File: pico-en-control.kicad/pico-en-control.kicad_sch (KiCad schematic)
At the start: 17 parts, among them J1 JST-PH2 Bat, J2 Pico Pin 1-13, J3 Pico Pin 40-28, SW1 SW_Push, U1 SN74HC74N, U2 PCF8563T, Y1 Crystal

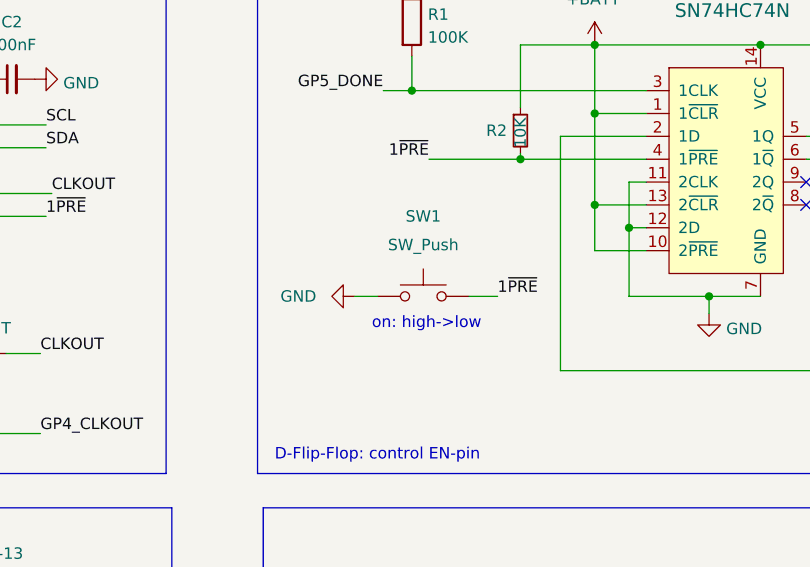
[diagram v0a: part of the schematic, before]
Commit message: Rev2
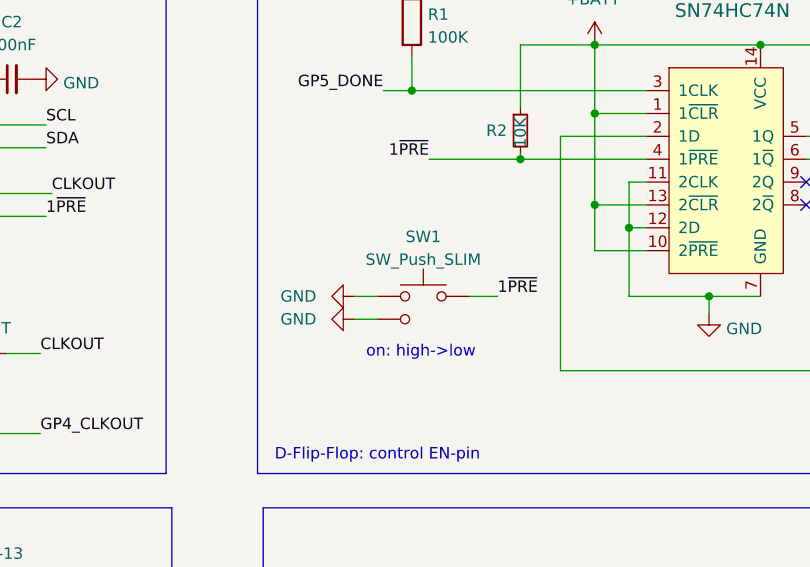
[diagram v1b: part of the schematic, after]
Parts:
- removed SW1: SW_Push, user:SW_PUSH_SLIM_1x4, symbol Switch:SW_Push
- added SW1: SW_Push_SLIM, user:SW_PUSH_SLIM_1x4, symbol user:SW_Push_SLIM
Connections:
- net 1~{PRE}: now also SW1.2
- net GND: now also SW1.1, SW1.3 (1)
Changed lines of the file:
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@@
+    (stroke (width 0) (type default) (color 0 0 0 0))
+  )
+  (wire (pts (xy 161.925 77.47) (xy 164.465 77.47))
     (stroke (width 0) (type default) (color 0 0 0 0))
   )
@@
     (effects (font (size 1.27 1.27)) (justify left bottom))
   )
-  (text "on: high->low" (at 163.83 78.74 0)
+  (text "on: high->low" (at 163.195 81.915 0)
     (effects (font (size 1.27 1.27)) (justify left bottom))
   )
@@
   (symbol (lib_id "power:GND") (at 123.825 137.795 90) (mirror x) (unit 1)
     (in_bom yes) (on_board yes)
-    (property "Reference" "#PWR?" (id 0) (at 130.175 137.795 0)
+    (property "Reference" "#PWR0107" (id 0) (at 130.175 137.795 0)
       (effects (font (size 1.27 1.27)) hide)
     )
@@
     (pin "1")
   )
+  (symbol (lib_id "power:GND") (at 161.925 77.47 270) (unit 1)
+    (in_bom yes) (on_board yes)
+    (property "Reference" "#PWR0110" (id 0) (at 155.575 77.47 0)
+      (effects (font (size 1.27 1.27)) hide)
+    )
+    (property "Value" "GND" (id 1) (at 153.67 77.47 90)
+      (effects (font (size 1.27 1.27)) (justify left))
+    )
+    (property "Footprint" "" (id 2) (at 161.925 77.47 0)
+      (effects (font (size 1.27 1.27)) hide)
+    )
+    (property "Datasheet" "" (id 3) (at 161.925 77.47 0)
+      (effects (font (size 1.27 1.27)) hide)
+    )
+    (pin "1")
+  )
   (symbol (lib_id "power:PWR_FLAG") (at 214.63 118.11 270) (unit 1)
     (in_bom yes) (on_board yes) (fields_autoplaced)
@@
   (symbol (lib_id "power:GND") (at 85.09 138.43 270) (unit 1)
     (in_bom yes) (on_board yes)
-    (property "Reference" "#PWR?" (id 0) (at 78.74 138.43 0)
+    (property "Reference" "#PWR0108" (id 0) (at 78.74 138.43 0)
       (effects (font (size 1.27 1.27)) hide)
     )
@@
     (pin "1")
   )
+  (symbol (lib_id "user:SW_Push_SLIM") (at 169.545 74.93 0) (unit 1)
+    (in_bom yes) (on_board yes) (fields_autoplaced)
+    (property "Reference" "SW1" (id 0) (at 169.545 68.3092 0))
+    (property "Value" "SW_Push_SLIM" (id 1) (at 169.545 70.8461 0))
+    (property "Footprint" "user:SW_PUSH_SLIM_1x4" (id 2) (at 169.545 82.55 0)
+      (effects (font (size 1.27 1.27)) hide)
+    )
+    (property "Datasheet" "" (id 3) (at 169.545 69.85 0)
+      (effects (font (size 1.27 1.27)) hide)
+    )
+    (pin "1")
+    (pin "2")
+    (pin "3")
+  )
   (symbol (lib_id "Device:C_Small") (at 218.44 46.99 90) (unit 1)
     (in_bom yes) (on_board yes)
@@
     )
     (property "LCSC" "C25744" (id 4) (at 90.17 82.55 0)
-      (effects (font (size 1.27 1.27)) hide)
-    )
-    (pin "1")
-    (pin "2")
-  )
-  (symbol (lib_id "Switch:SW_Push") (at 169.545 74.93 0) (unit 1)
-    (in_bom yes) (on_board yes)
-    (property "Reference" "SW1" (id 0) (at 169.545 66.04 0))
-    (property "Value" "SW_Push" (id 1) (at 169.545 69.215 0))
-    (property "Footprint" "user:SW_PUSH_SLIM_1x4" (id 2) (at 169.545 69.85 0)
-      (effects (font (size 1.27 1.27)) hide)
-    )
-    (property "Datasheet" "~" (id 3) (at 169.545 69.85 0)
       (effects (font (size 1.27 1.27)) hide)
     )
@@
   (symbol (lib_id "power:GND") (at 85.09 125.73 270) (unit 1)
     (in_bom yes) (on_board yes)
-    (property "Reference" "#PWR?" (id 0) (at 78.74 125.73 0)
+    (property "Reference" "#PWR0109" (id 0) (at 78.74 125.73 0)
       (effects (font (size 1.27 1.27)) hide)
     )
@@
   (symbol (lib_id "power:GND") (at 123.825 125.095 90) (mirror x) (unit 1)
     (in_bom yes) (on_board yes)
-    (property "Reference" "#PWR?" (id 0) (at 130.175 125.095 0)
+    (property "Reference" "#PWR0106" (id 0) (at 130.175 125.095 0)
       (effects (font (size 1.27 1.27)) hide)
     )
@@
       (reference "#PWR0105") (unit 1) (value "+3V3") (footprint "")
     )
+    (path "/da0d7de8-a385-4e20-96bb-738a9abcf740"
+      (reference "#PWR0106") (unit 1) (value "GND") (footprint "")
+    )
     (path "/2721609c-f161-4649-8caf-b27c7748cbdb"
-      (reference "#PWR?") (unit 1) (value "GND") (footprint "")
+      (reference "#PWR0107") (unit 1) (value "GND") (footprint "")
     )
     (path "/3e266c6d-5aba-467c-9ae1-a13ae4e195a5"
-      (reference "#PWR?") (unit 1) (value "GND") (footprint "")
+      (reference "#PWR0108") (unit 1) (value "GND") (footprint "")
     )
     (path "/9daade84-f146-4e38-9889-9c3ac72475f9"
-      (reference "#PWR?") (unit 1) (value "GND") (footprint "")
-    )
-    (path "/da0d7de8-a385-4e20-96bb-738a9abcf740"
-      (reference "#PWR?") (unit 1) (value "GND") (footprint "")
+      (reference "#PWR0109") (unit 1) (value "GND") (footprint "")
+    )
+    (path "/34aa5534-e445-4f46-8589-62223cf8ef18"
+      (reference "#PWR0110") (unit 1) (value "GND") (footprint "")
     )
     (path "/5bee97ec-80e1-4be7-a685-5921db869610"
@@
       (reference "R5") (unit 1) (value "10K") (footprint "Resistor_SMD:R_0402_1005Metric")
     )
-    (path "/8eb4a059-c6b6-4dfe-acee-59cf9f265db1"
-      (reference "SW1") (unit 1) (value "SW_Push") (footprint "user:SW_PUSH_SLIM_1x4")
+    (path "/58a4b577-49cb-4d3a-a75f-433d25045363"
+      (reference "SW1") (unit 1) (value "SW_Push_SLIM") (footprint "user:SW_PUSH_SLIM_1x4")
     )
     (path "/aeee191c-38fd-4ab0-b212-9eafb9d35bdc"
